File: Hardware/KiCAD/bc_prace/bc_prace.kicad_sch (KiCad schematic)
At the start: 0 parts

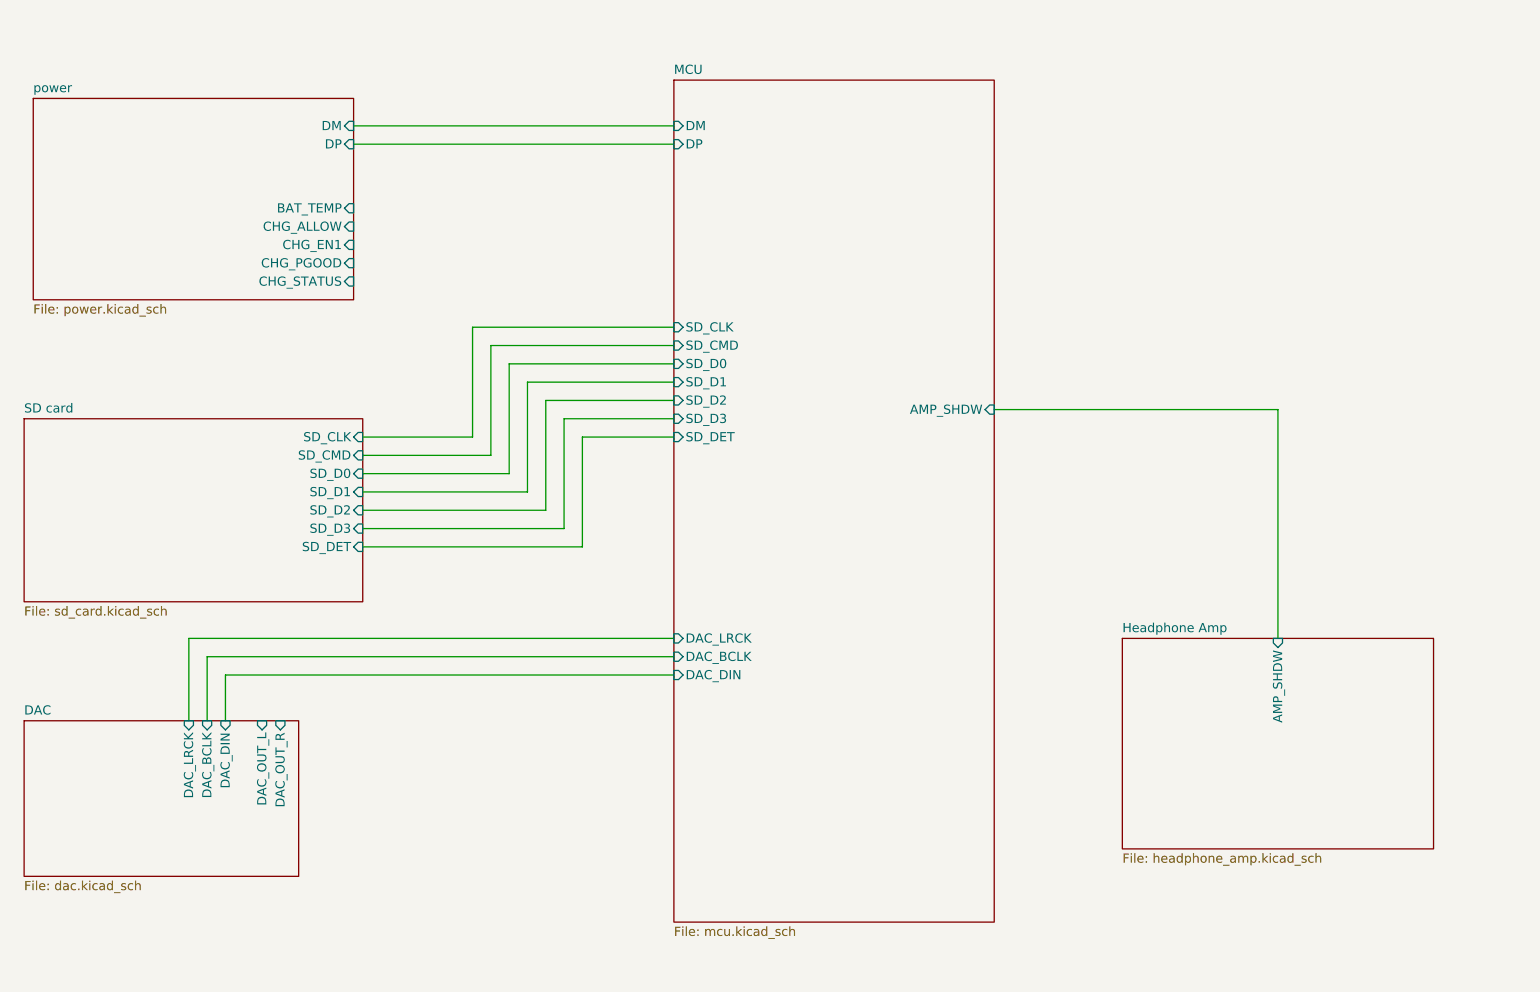
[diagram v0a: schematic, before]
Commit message: kicad
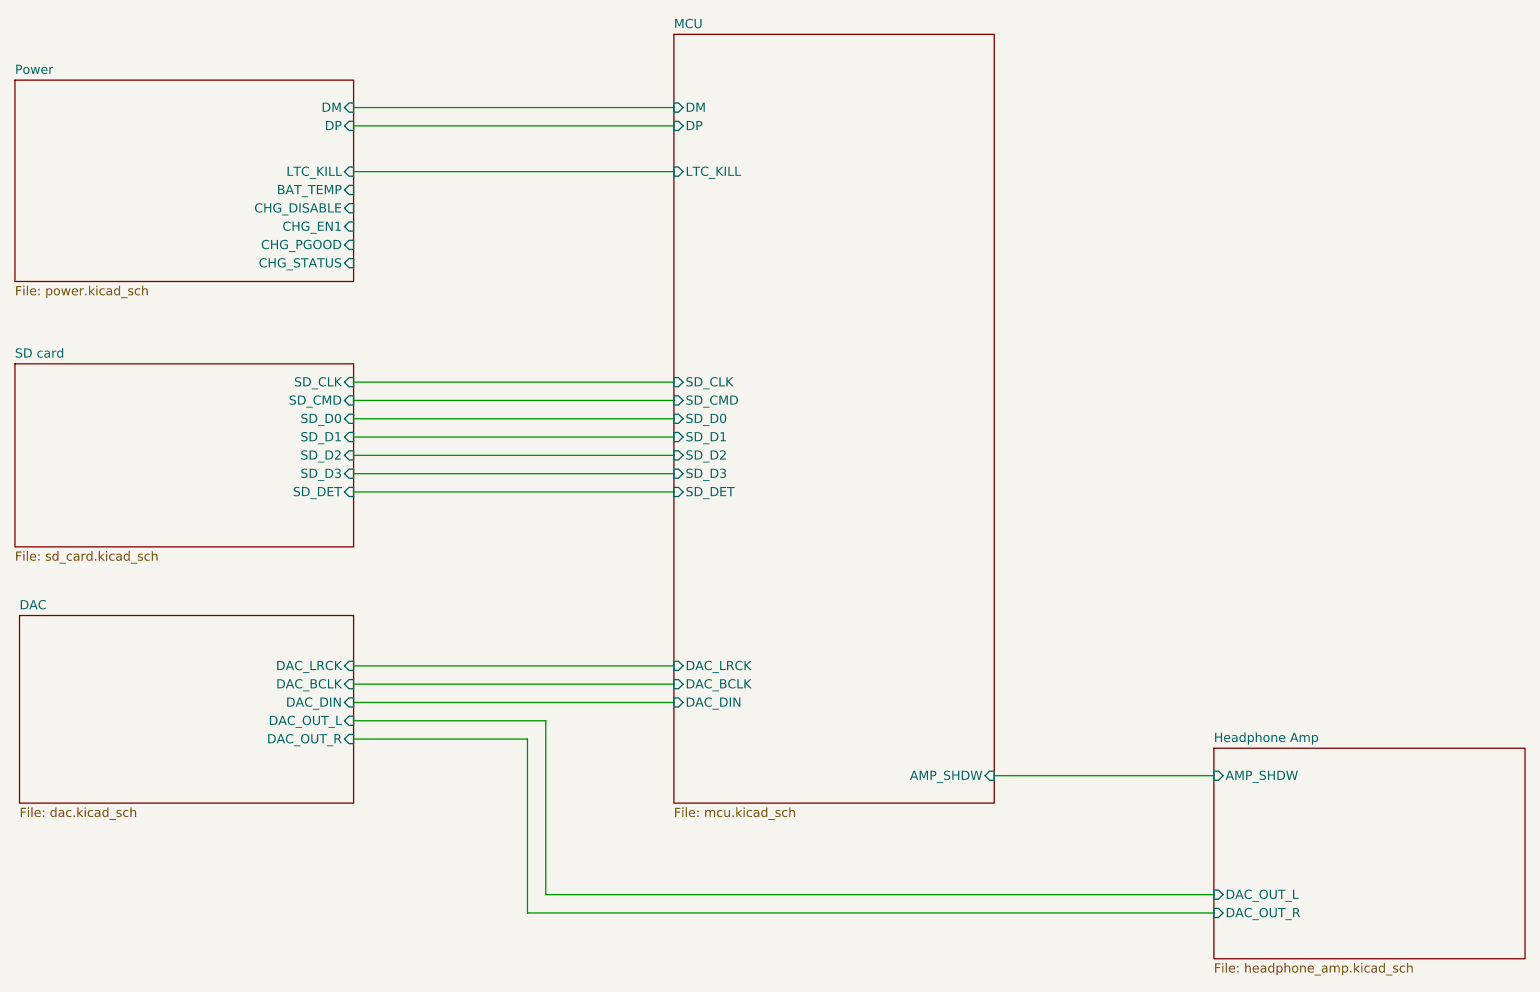
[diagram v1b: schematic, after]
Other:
- sheet power renamed Power
- sheet Headphone Amp ports: added DAC_OUT_L, DAC_OUT_R; removed none
- sheet MCU ports: added LTC_KILL; removed none
- sheet Power ports: added CHG_DISABLE, LTC_KILL; removed CHG_ALLOW
